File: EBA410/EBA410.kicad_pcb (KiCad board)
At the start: 2 copper layers, 42 x 25 mm, 3 parts, among them P1 rt, P2 auf L-SEITE

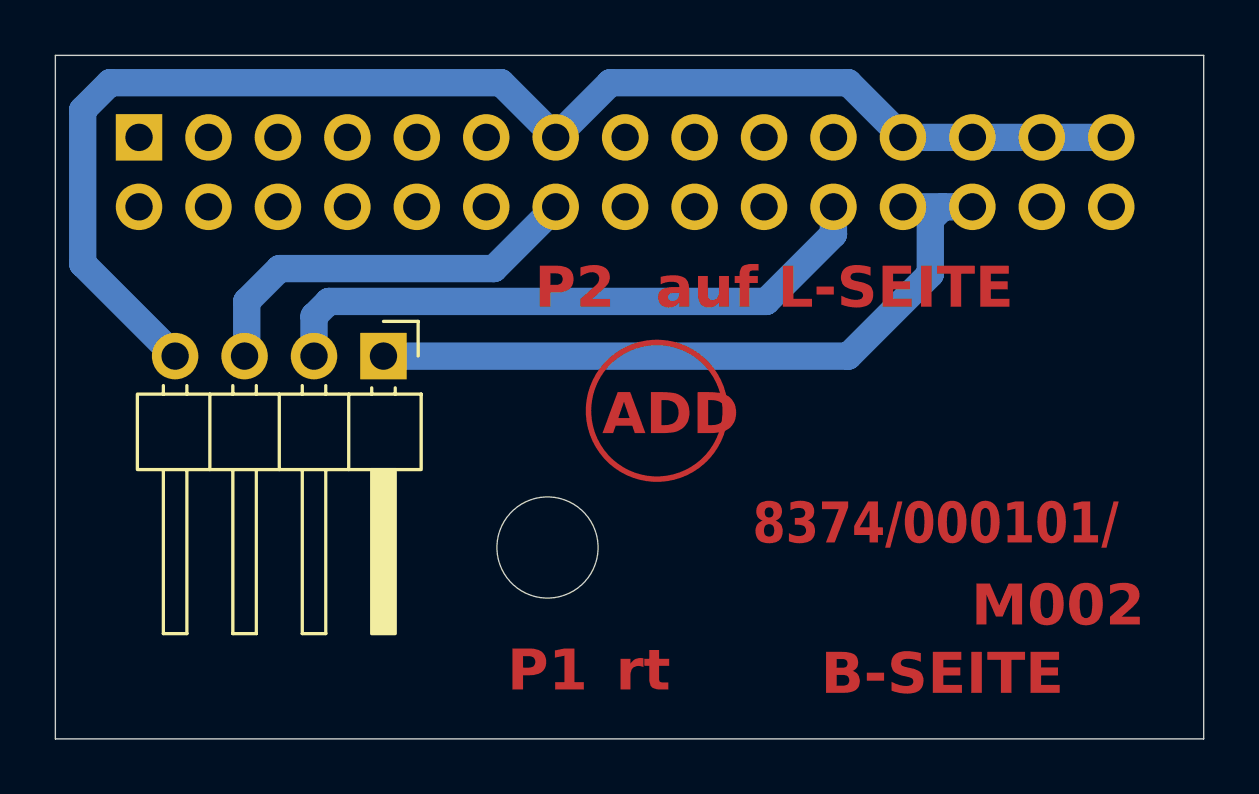
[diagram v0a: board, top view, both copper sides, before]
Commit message: ercdrc
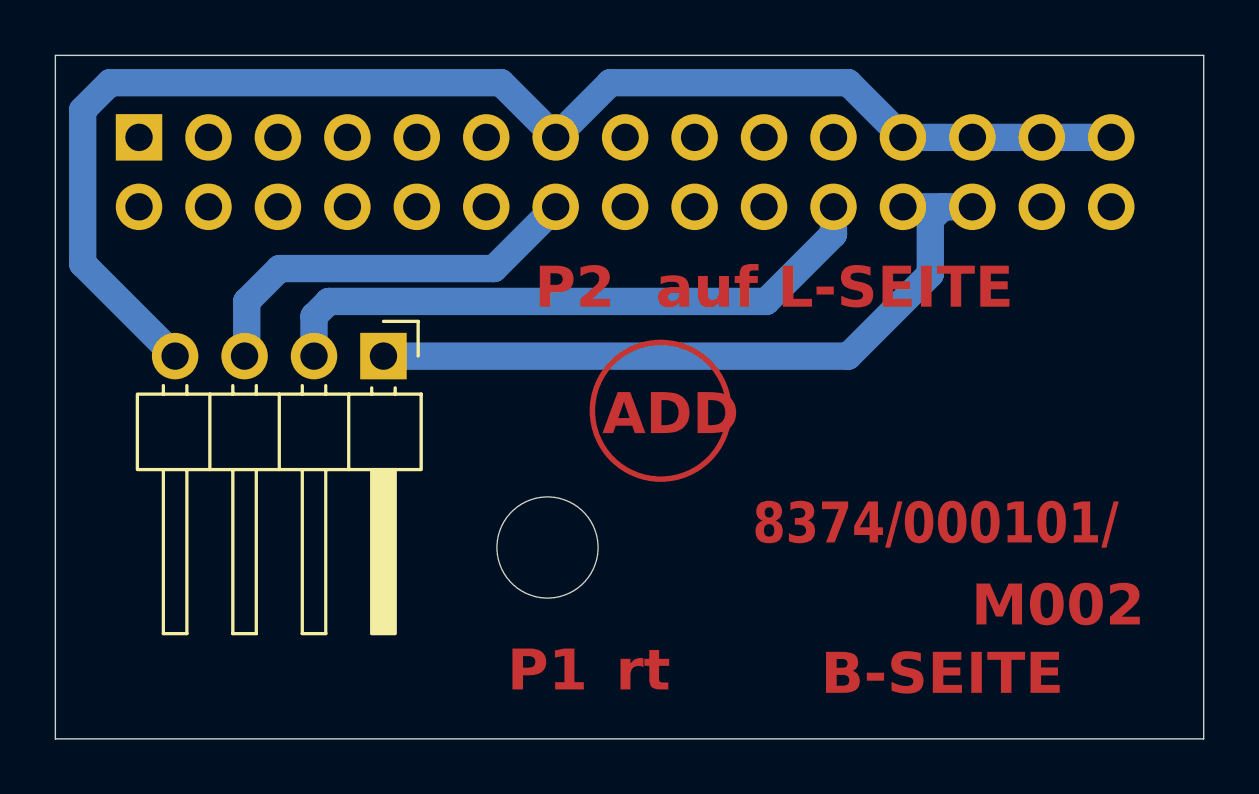
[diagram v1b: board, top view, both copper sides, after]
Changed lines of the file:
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@@
 			(net 21 "unconnected-(P2-Pin_1-Pad1)")
 			(pinfunction "Pin_1")
-			(pintype "passive")
+			(pintype "passive+no_connect")
 		)
 		(pad "2" thru_hole circle
@@
 			(net 10 "unconnected-(P2-Pin_2-Pad2)")
 			(pinfunction "Pin_2")
-			(pintype "passive")
+			(pintype "passive+no_connect")
 		)
 		(pad "3" thru_hole circle
@@
 			(net 15 "unconnected-(P2-Pin_3-Pad3)")
 			(pinfunction "Pin_3")
-			(pintype "passive")
+			(pintype "passive+no_connect")
 		)
 		(pad "4" thru_hole circle
@@
 			(net 5 "unconnected-(P2-Pin_4-Pad4)")
 			(pinfunction "Pin_4")
-			(pintype "passive")
+			(pintype "passive+no_connect")
 		)
 		(pad "5" thru_hole circle
@@
 			(net 14 "unconnected-(P2-Pin_5-Pad5)")
 			(pinfunction "Pin_5")
-			(pintype "passive")
+			(pintype "passive+no_connect")
 		)
 		(pad "6" thru_hole circle
@@
 			(net 11 "unconnected-(P2-Pin_6-Pad6)")
 			(pinfunction "Pin_6")
-			(pintype "passive")
+			(pintype "passive+no_connect")
 		)
 		(pad "7" thru_hole circle
@@
 			(net 25 "unconnected-(P2-Pin_7-Pad7)")
 			(pinfunction "Pin_7")
-			(pintype "passive")
+			(pintype "passive+no_connect")
 		)
 		(pad "8" thru_hole circle
@@
 			(net 18 "unconnected-(P2-Pin_8-Pad8)")
 			(pinfunction "Pin_8")
-			(pintype "passive")
+			(pintype "passive+no_connect")
 		)
 		(pad "9" thru_hole circle
@@
 			(net 6 "unconnected-(P2-Pin_9-Pad9)")
 			(pinfunction "Pin_9")
-			(pintype "passive")
+			(pintype "passive+no_connect")
 		)
 		(pad "10" thru_hole circle
@@
 			(net 19 "unconnected-(P2-Pin_10-Pad10)")
 			(pinfunction "Pin_10")
-			(pintype "passive")
+			(pintype "passive+no_connect")
 		)
 		(pad "11" thru_hole circle
@@
 			(net 16 "unconnected-(P2-Pin_11-Pad11)")
 			(pinfunction "Pin_11")
-			(pintype "passive")
+			(pintype "passive+no_connect")
 		)
 		(pad "12" thru_hole circle
@@
 			(net 24 "unconnected-(P2-Pin_12-Pad12)")
 			(pinfunction "Pin_12")
-			(pintype "passive")
+			(pintype "passive+no_connect")
 		)
 		(pad "13" thru_hole circle
@@
 			(net 22 "unconnected-(P2-Pin_15-Pad15)")
 			(pinfunction "Pin_15")
-			(pintype "passive")
+			(pintype "passive+no_connect")
 		)
 		(pad "16" thru_hole circle
@@
 			(net 9 "unconnected-(P2-Pin_16-Pad16)")
 			(pinfunction "Pin_16")
-			(pintype "passive")
+			(pintype "passive+no_connect")
 		)
 		(pad "17" thru_hole circle
@@
 			(net 20 "unconnected-(P2-Pin_17-Pad17)")
 			(pinfunction "Pin_17")
-			(pintype "passive")
+			(pintype "passive+no_connect")
 		)
 		(pad "18" thru_hole circle
@@
 			(net 8 "unconnected-(P2-Pin_18-Pad18)")
 			(pinfunction "Pin_18")
-			(pintype "passive")
+			(pintype "passive+no_connect")
 		)
 		(pad "19" thru_hole circle
@@
 			(net 17 "unconnected-(P2-Pin_19-Pad19)")
 			(pinfunction "Pin_19")
-			(pintype "passive")
+			(pintype "passive+no_connect")
 		)
 		(pad "20" thru_hole circle
@@
 			(net 12 "unconnected-(P2-Pin_20-Pad20)")
 			(pinfunction "Pin_20")
-			(pintype "passive")
+			(pintype "passive+no_connect")
 		)
 		(pad "21" thru_hole circle
@@
 			(net 23 "unconnected-(P2-Pin_21-Pad21)")
 			(pinfunction "Pin_21")
-			(pintype "passive")
+			(pintype "passive+no_connect")
 		)
 		(pad "22" thru_hole circle
@@
 			(net 7 "unconnected-(P2-Pin_28-Pad28)")
 			(pinfunction "Pin_28")
-			(pintype "passive")
+			(pintype "passive+no_connect")
 		)
 		(pad "29" thru_hole circle
@@
 			(net 13 "unconnected-(P2-Pin_30-Pad30)")
 			(pinfunction "Pin_30")
-			(pintype "passive")
+			(pintype "passive+no_connect")
 		)
 		(embedded_fonts no)
@@
 	)
 	(gr_circle
-		(center 120 71)
-		(end 122.5 71)
+		(center 120.142 71)
+		(end 122.642 71)
 		(stroke
 			(width 0.2)
@@
 		)
 	)
+	(gr_text "8374/000101/"
+		(at 123.5 76 0)
+		(layer "F.Cu")
+		(effects
+			(font
+				(size 1.5 1.27)
+				(thickness 0.3)
+				(bold yes)
+			)
+			(justify left bottom)
+		)
+	)
 	(gr_text "ADD"
 		(at 118 72 0)
@@
 		)
 	)
-	(gr_text "8374/000101/"
-		(at 123.5 76 0)
-		(layer "F.Cu")
-		(effects
-			(font
-				(size 1.5 1.27)
-				(thickness 0.3)
-				(bold yes)
-			)
-			(justify left bottom)
-		)
-	)
-	(gr_text "M002"
-		(at 131.5 79 0)
+	(gr_text "B-SEITE"
+		(at 126 81.5 0)
 		(layer "F.Cu")
 		(effects
@@
 		)
 	)
-	(gr_text "B-SEITE"
-		(at 126 81.5 0)
+	(gr_text "M002"
+		(at 131.5 79 0)
 		(layer "F.Cu")
 		(effects
